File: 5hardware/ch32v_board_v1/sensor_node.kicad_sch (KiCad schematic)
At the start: 19 parts, among them J1 Conn_01x06_Pin, J2 Conn_01x08_Pin, J3 Conn_01x09_Pin, J4 USB_C_Receptacle_USB2.0, J5 Conn_01x09_Pin, SW1 SW_Push, U2 CH32V003F4P6, U3 XC6206PxxxMR

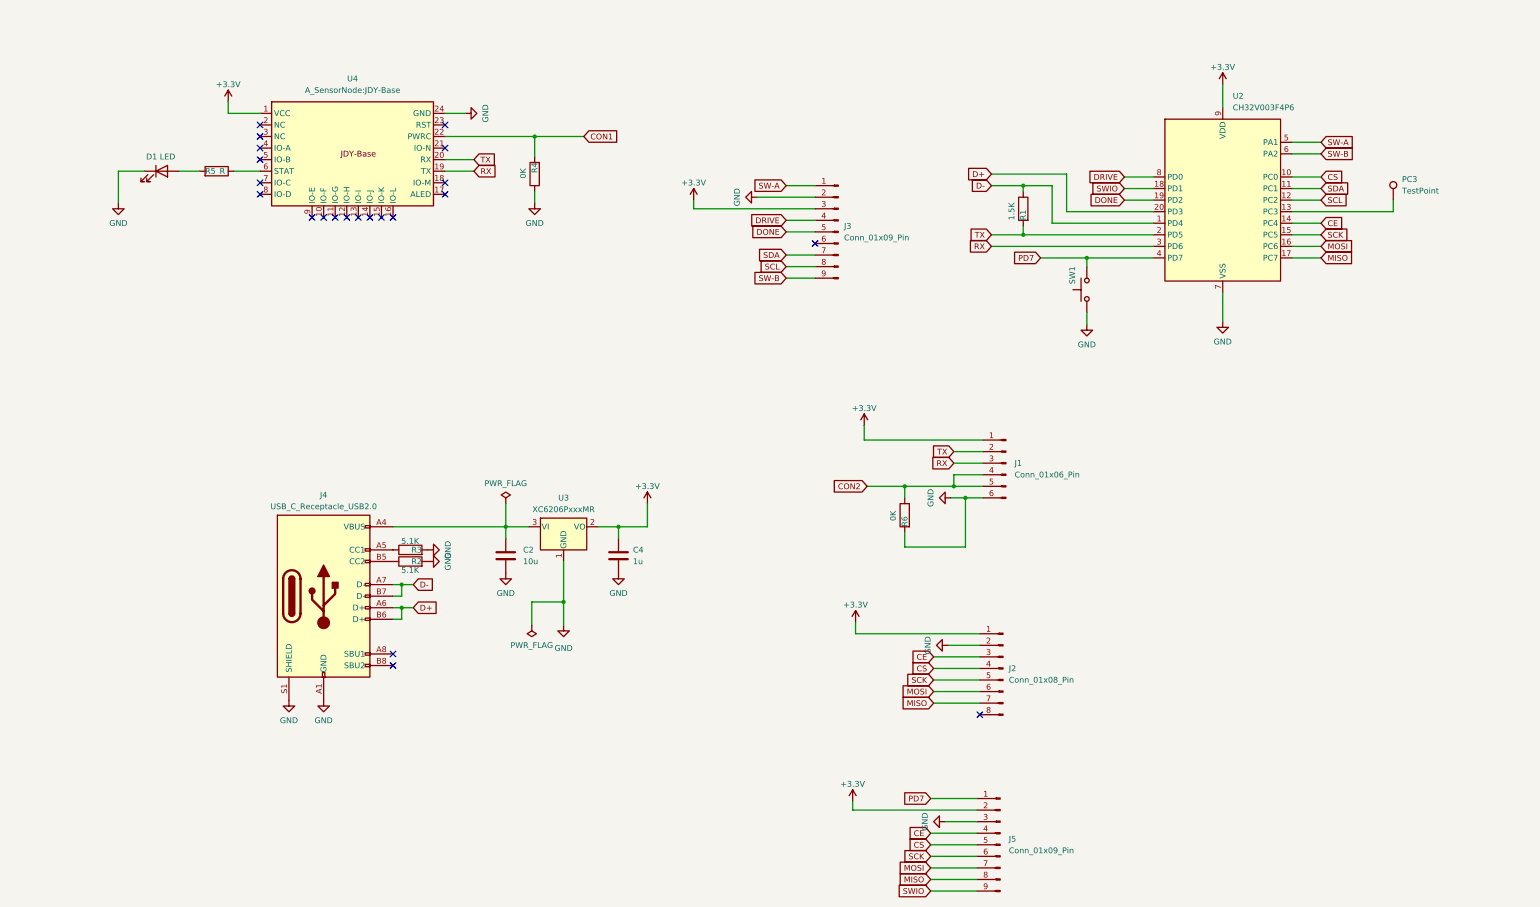
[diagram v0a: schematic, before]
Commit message: udpate PCBs.
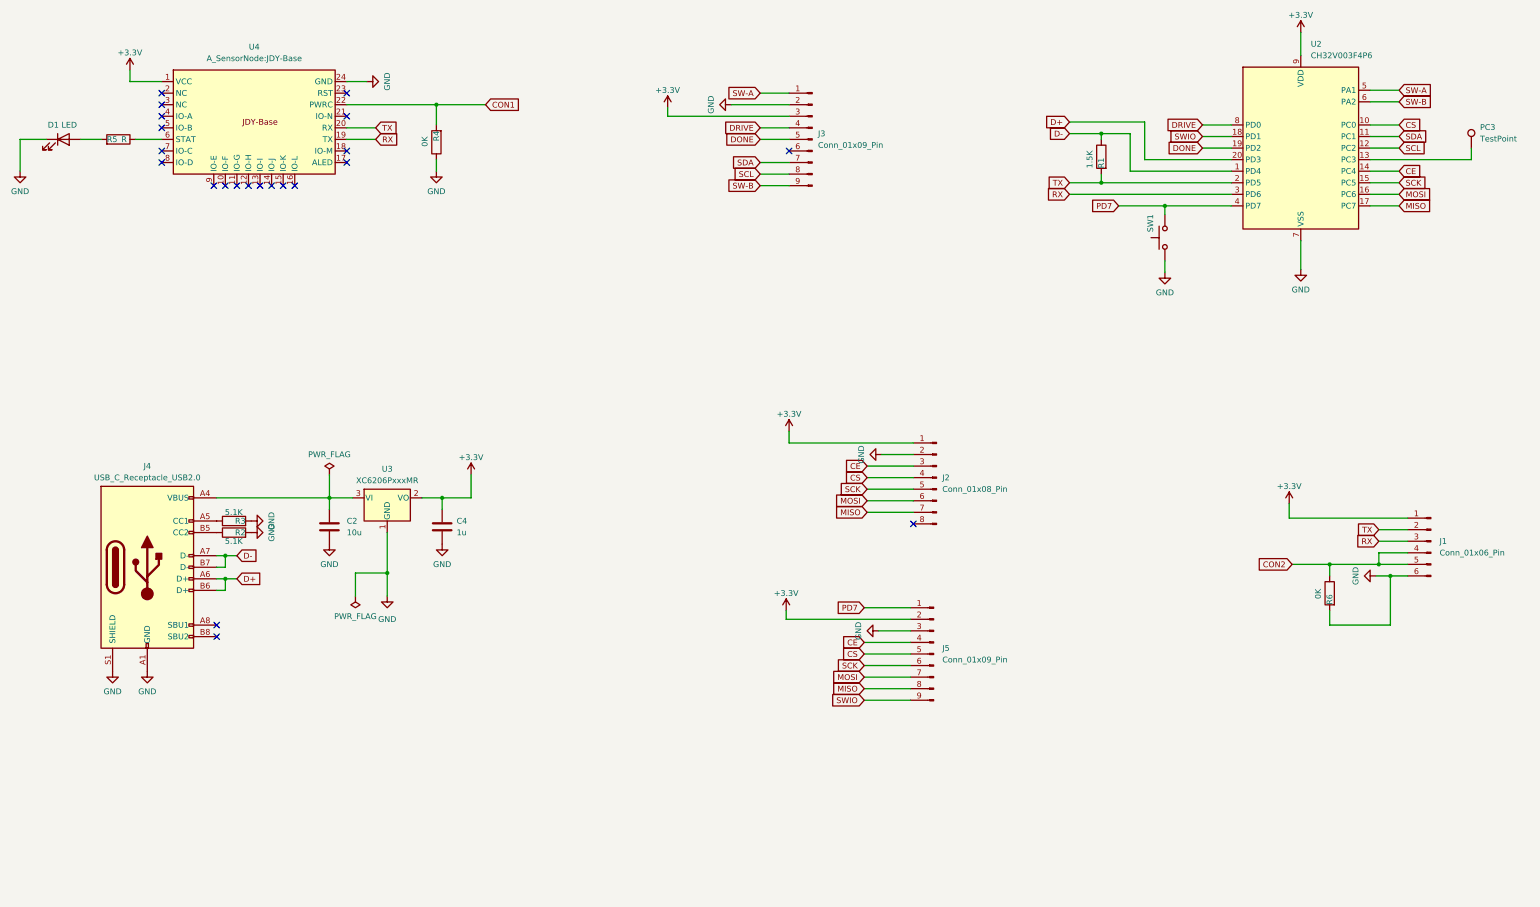
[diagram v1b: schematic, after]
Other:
- moved on the sheet: C2, C4, D1, J1, J2, J3, J4, J5, PC3, R1, R2, R3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
